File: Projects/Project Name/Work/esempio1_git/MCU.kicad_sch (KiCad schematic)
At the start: 38 parts, among them J1 Conn_01x06, J2 Conn_01x03, J3 Conn_01x08, SW1 SW_DIP_x01, U1 STM32F405RGTx, Y1 Crystal

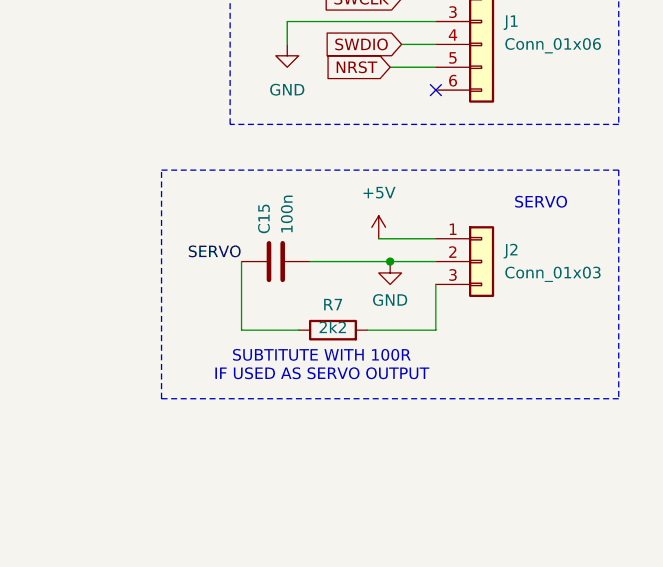
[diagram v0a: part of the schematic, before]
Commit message: Update 2
Aggiunta MosfetDriver
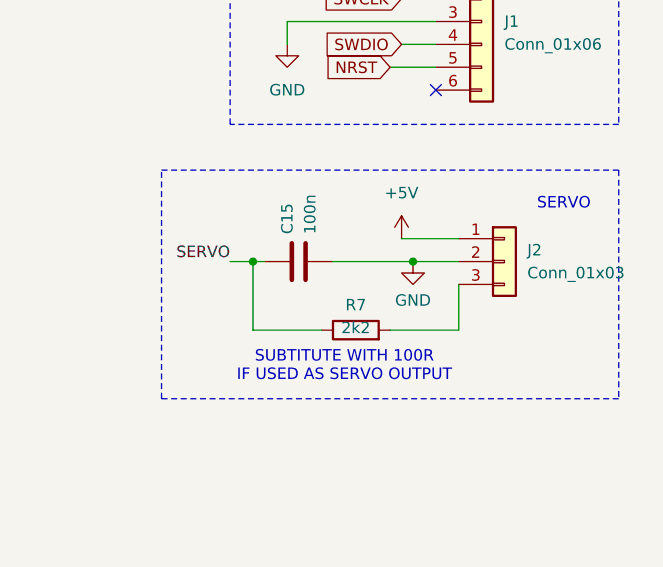
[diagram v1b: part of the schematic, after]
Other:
- moved on the sheet: C15, J2, R7
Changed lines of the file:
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@@
 	)
 	(junction
-		(at 246.38 121.92)
+		(at 248.92 121.92)
 		(diameter 0)
 		(color 0 0 0 0)
@@
 	)
 	(junction
+		(at 231.14 121.92)
+		(diameter 0)
+		(color 0 0 0 0)
+	)
+	(junction
 		(at 250.19 40.64)
 		(diameter 0)
@@
 	(wire
 		(pts
-			(xy 246.38 121.92) (xy 251.46 121.92)
+			(xy 248.92 121.92) (xy 254 121.92)
 		)
 		(stroke
@@
 	(wire
 		(pts
-			(xy 237.49 121.92) (xy 246.38 121.92)
+			(xy 240.03 121.92) (xy 248.92 121.92)
 		)
 		(stroke
@@
 	(wire
 		(pts
+			(xy 228.6 121.92) (xy 231.14 121.92)
+		)
+		(stroke
+			(width 0)
+			(type default)
+		)
+	)
+	(wire
+		(pts
 			(xy 173.99 129.54) (xy 176.53 129.54)
 		)
@@
 	(wire
 		(pts
-			(xy 251.46 129.54) (xy 243.84 129.54)
+			(xy 254 129.54) (xy 246.38 129.54)
 		)
 		(stroke
@@
 	(wire
 		(pts
-			(xy 251.46 124.46) (xy 251.46 129.54)
+			(xy 254 124.46) (xy 254 129.54)
 		)
 		(stroke
@@
 	(wire
 		(pts
-			(xy 229.87 129.54) (xy 229.87 121.92)
+			(xy 231.14 129.54) (xy 231.14 121.92)
 		)
 		(stroke
@@
 	(wire
 		(pts
-			(xy 245.11 119.38) (xy 251.46 119.38)
+			(xy 247.65 119.38) (xy 254 119.38)
 		)
 		(stroke
@@
 	(wire
 		(pts
-			(xy 236.22 129.54) (xy 229.87 129.54)
+			(xy 238.76 129.54) (xy 231.14 129.54)
 		)
 		(stroke
@@
 	(wire
 		(pts
+			(xy 231.14 121.92) (xy 232.41 121.92)
+		)
+		(stroke
+			(width 0)
+			(type default)
+		)
+	)
+	(wire
+		(pts
 			(xy 44.45 34.29) (xy 52.07 34.29)
 		)
@@
 	(text "SERVO"
 		(exclude_from_sim no)
-		(at 263.144 115.57 0)
+		(at 265.684 115.57 0)
 		(effects
 			(font
@@
 	(text "SUBTITUTE WITH 100R\nIF USED AS SERVO OUTPUT"
 		(exclude_from_sim no)
-		(at 238.76 133.604 0)
+		(at 241.3 133.604 0)
 		(effects
 			(font
@@
 	)
 	(label "SERVO"
-		(at 229.87 121.92 180)
+		(at 228.6 121.92 180)
 		(effects
 			(font
@@
 	(symbol
 		(lib_id "Device:R")
-		(at 240.03 129.54 90)
+		(at 242.57 129.54 90)
 		(unit 1)
 		(exclude_from_sim no)
@@
 		(dnp no)
 		(property "Reference" "R7"
-			(at 240.03 126.746 90)
+			(at 242.57 126.746 90)
 			(effects
 				(font
@@
 		)
 		(property "Value" "2k2"
-			(at 240.03 129.286 90)
+			(at 242.57 129.286 90)
 			(effects
 				(font
@@
 		)
 		(property "Footprint" ""
-			(at 240.03 131.318 90)
+			(at 242.57 131.318 90)
 			(effects
 				(font
@@
 		)
 		(property "Datasheet" "~"
-			(at 240.03 129.54 0)
+			(at 242.57 129.54 0)
 			(effects
 				(font
@@
 		)
 		(property "Description" "Resistor"
-			(at 240.03 129.54 0)
+			(at 242.57 129.54 0)
 			(effects
 				(font
@@
 	(symbol
 		(lib_id "power:GND")
-		(at 246.38 121.92 0)
+		(at 248.92 121.92 0)
 		(unit 1)
 		(exclude_from_sim no)
@@
 		(dnp no)
 		(property "Reference" "#PWR016"
-			(at 246.38 128.27 0)
+			(at 248.92 128.27 0)
 			(effects
 				(font
@@
 		)
 		(property "Value" "GND"
-			(at 246.38 126.238 0)
+			(at 248.92 126.238 0)
 			(effects
 				(font
@@
 		)
 		(property "Footprint" ""
-			(at 246.38 121.92 0)
+			(at 248.92 121.92 0)
 			(effects
 				(font
@@
 		)
 		(property "Datasheet" ""
-			(at 246.38 121.92 0)
+			(at 248.92 121.92 0)
 			(effects
 				(font
@@
 		)
 		(property "Description" "Power symbol creates a global label with name \"GND\" , ground"
-			(at 246.38 121.92 0)
+			(at 248.92 121.92 0)
 			(effects
 				(font
@@
 	(symbol
 		(lib_id "Connector_Generic:Conn_01x03")
-		(at 256.54 121.92 0)
+		(at 259.08 121.92 0)
 		(unit 1)
 		(exclude_from_sim no)
@@
 		(fields_autoplaced yes)
 		(property "Reference" "J2"
-			(at 259.08 120.6499 0)
+			(at 261.62 120.6499 0)
 			(effects
 				(font
@@
 		)
 		(property "Value" "Conn_01x03"
-			(at 259.08 123.1899 0)
+			(at 261.62 123.1899 0)
 			(effects
 				(font
@@
 		)
 		(property "Footprint" ""
-			(at 256.54 121.92 0)
+			(at 259.08 121.92 0)
 			(effects
 				(font
@@
 		)
 		(property "Datasheet" "~"
-			(at 256.54 121.92 0)
+			(at 259.08 121.92 0)
 			(effects
 				(font
@@
 		)
 		(property "Description" "Generic connector, single row, 01x03, script generated (kicad-library-utils/schlib/autogen/connector/)"
-			(at 256.54 121.92 0)
+			(at 259.08 121.92 0)
 			(effects
 				(font
@@
 	(symbol
 		(lib_id "power:+5V")
-		(at 245.11 119.38 0)
+		(at 247.65 119.38 0)
 		(unit 1)
 		(exclude_from_sim no)
@@
 		(fields_autoplaced yes)
 		(property "Reference" "#PWR015"
-			(at 245.11 123.19 0)
+			(at 247.65 123.19 0)
 			(effects
 				(font
@@
 		)
 		(property "Value" "+5V"
-			(at 245.11 114.3 0)
+			(at 247.65 114.3 0)
 			(effects
 				(font
@@
 		)
 		(property "Footprint" ""
-			(at 245.11 119.38 0)
+			(at 247.65 119.38 0)
 			(effects
 				(font
@@
 		)
 		(property "Datasheet" ""
-			(at 245.11 119.38 0)
+			(at 247.65 119.38 0)
 			(effects
 				(font
@@
 		)
 		(property "Description" "Power symbol creates a global label with name \"+5V\""
-			(at 245.11 119.38 0)
+			(at 247.65 119.38 0)
 			(effects
 				(font
@@
 	(symbol
 		(lib_id "Device:C")
-		(at 233.68 121.92 90)
+		(at 236.22 121.92 90)
 		(unit 1)
 		(exclude_from_sim no)
@@
 		(dnp no)
 		(property "Reference" "C15"
-			(at 232.41 118.872 0)
+			(at 234.95 118.872 0)
 			(effects
 				(font
@@
 		)
 		(property "Value" "100n"
-			(at 234.95 118.872 0)
+			(at 237.49 118.872 0)
 			(effects
 				(font
@@
 		)
 		(property "Footprint" ""
-			(at 237.49 120.9548 0)
+			(at 240.03 120.9548 0)
 			(effects
 				(font
@@
 		)
 		(property "Datasheet" "~"
-			(at 233.68 121.92 0)
+			(at 236.22 121.92 0)
 			(effects
 				(font
@@
 		)
 		(property "Description" "Unpolarized capacitor"
-			(at 233.68 121.92 0)
+			(at 236.22 121.92 0)
 			(effects
 				(font
